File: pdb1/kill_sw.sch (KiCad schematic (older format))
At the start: 7 parts, among them P4 CONN_02X03, Q2 BUK9Y4R8-60E, U7 MIC5014, U8 NSI45020AT1G

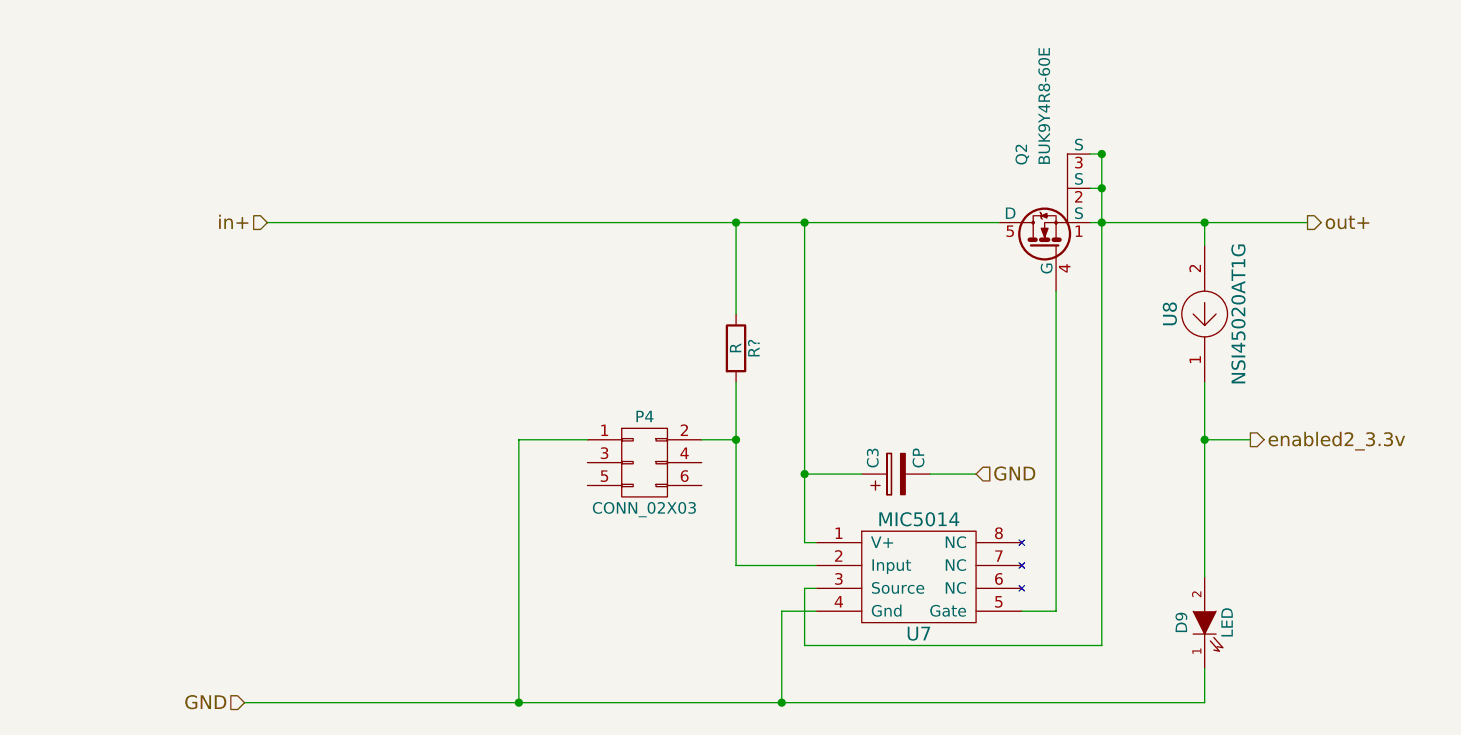
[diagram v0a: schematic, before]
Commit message: test
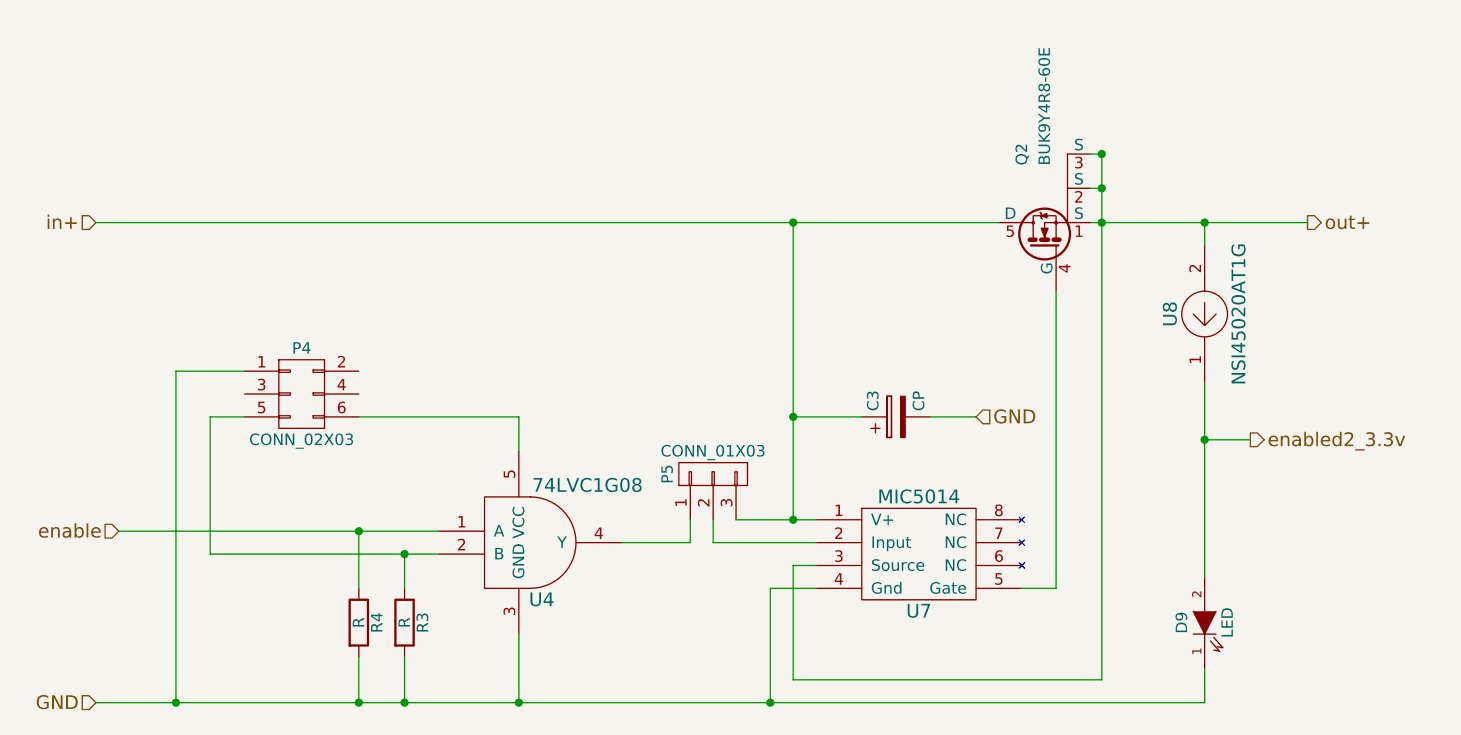
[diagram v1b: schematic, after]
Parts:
- removed R?: R, symbol R
- added P5: CONN_01X03, Pin_Headers:Pin_Header_Straight_1x03, symbol CONN_01X03
- added R3, R4: R, Resistors_SMD:R_0603, symbol R
- added U4: 74LVC1G08, TO_SOT_Packages_SMD:SOT-353, symbol 74LVC1G08
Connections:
- net GND: now also R3.2, R4.2, U4.3 (GND)
- net in+: now also P5.3 (P3)
- net at U7.2 (Input): now also P5.2 (P2); no longer P4.2 (P2)
- net at P4.5 (P5): now also R3.1, U4.2 (B)
- net at P4.6 (P6): now also U4.5 (VCC)
- new net: P5.1 (P1), U4.4 (Y)
- new net enable: R4.1, U4.1 (A)
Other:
- moved on the sheet: C3, P4, U7
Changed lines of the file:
@@
 L MIC5014 U?
 U 1 1 581F4598
-P 5250 4200
+P 5250 4100
 AR Path="/581F28FF/581F4598" Ref="U?"  Part="1"
 AR Path="/581FE101/581FE98D/581F4598" Ref="U7"  Part="1"
-F 0 "U7" H 5250 3950 60  0000 C CNN
-F 1 "MIC5014" H 5250 4450 60  0000 C CNN
-F 2 "Housings_SOIC:SOIC-8_3.9x4.9mm_Pitch1.27mm" H 5250 4100 60  0001 C CNN
-F 3 "http://www.farnell.com/datasheets/29565.pdf" H 5250 3850 60  0001 C CNN
-	1    5250 4200
-	1    0    0    -1
-$EndComp
-Text HLabel 2400 2650 0    60   Input ~ 0
+F 0 "U7" H 5250 3850 60  0000 C CNN
+F 1 "MIC5014" H 5250 4350 60  0000 C CNN
+F 2 "Housings_SOIC:SOIC-8_3.9x4.9mm_Pitch1.27mm" H 5250 4000 60  0001 C CNN
+F 3 "http://www.farnell.com/datasheets/29565.pdf" H 5250 3750 60  0001 C CNN
+	1    5250 4100
+	1    0    0    -1
+$EndComp
+Text HLabel 1650 2650 0    60   Input ~ 0
 in+
-Text HLabel 2300 4750 0    60   Input ~ 0
+Text HLabel 1650 4750 0    60   Input ~ 0
 GND
 Text HLabel 6950 2650 2    60   Output ~ 0
@@
 	0    -1   -1   0
 $EndComp
-Wire Wire Line
-	4750 4050 4800 4050
-Wire Wire Line
-	4750 2650 4750 4050
-Wire Wire Line
-	2400 2650 5600 2650
-Connection ~ 4750 2650
-Wire Wire Line
-	5850 2950 5850 4350
-Wire Wire Line
-	5850 4350 5700 4350
-Wire Wire Line
-	4650 4750 4650 4350
-Wire Wire Line
-	4650 4350 4800 4350
-Connection ~ 4650 4750
-Wire Wire Line
-	6000 2650 6950 2650
-Wire Wire Line
-	4800 4250 4750 4250
-Wire Wire Line
-	4750 4250 4750 4500
-Wire Wire Line
-	4750 4500 6050 4500
-Connection ~ 6050 2650
-Connection ~ 4750 3750
-Connection ~ 3500 4750
-Wire Wire Line
-	6500 2750 6500 2650
-Connection ~ 6500 2650
-Wire Wire Line
-	6500 4750 6500 4600
-Wire Wire Line
-	6500 3350 6500 4200
-Wire Wire Line
-	4750 3750 5000 3750
-Wire Wire Line
-	5300 3750 5500 3750
 Text HLabel 6700 3600 2    60   Output ~ 0
 enabled2_3.3v
-Wire Wire Line
-	6700 3600 6500 3600
-Connection ~ 6500 3600
-Wire Wire Line
-	2300 4750 6500 4750
-Text HLabel 5500 3750 2    60   Input ~ 0
+Text HLabel 5500 3500 2    60   Input ~ 0
 GND
 $Comp
@@
 	0    -1   -1   0
 $EndComp
+$Comp
+L CP C3
+U 1 1 5825B68F
+P 5150 3500
+F 0 "C3" H 5175 3600 50  0000 L CNN
+F 1 "CP" H 5175 3400 50  0000 L CNN
+F 2 "Capacitors_ThroughHole:C_Radial_D5_L6_P2.5" H 5188 3350 50  0001 C CNN
+F 3 "" H 5150 3500 50  0000 C CNN
+	1    5150 3500
+	0    -1   -1   0
+$EndComp
+$Comp
+L CONN_02X03 P4
+U 1 1 5825EF78
+P 2550 3400
+F 0 "P4" H 2550 3600 50  0000 C CNN
+F 1 "CONN_02X03" H 2550 3200 50  0000 C CNN
+F 2 "Pin_Headers:Pin_Header_Straight_2x03" H 2550 2200 50  0001 C CNN
+F 3 "" H 2550 2200 50  0000 C CNN
+	1    2550 3400
+	1    0    0    -1
+$EndComp
+$Comp
+L R R3
+U 1 1 582707A5
+P 3000 4400
+F 0 "R3" V 3080 4400 50  0000 C CNN
+F 1 "R" V 3000 4400 50  0000 C CNN
+F 2 "Resistors_SMD:R_0603" V 2930 4400 50  0001 C CNN
+F 3 "" H 3000 4400 50  0000 C CNN
+	1    3000 4400
+	1    0    0    -1
+$EndComp
+$Comp
+L 74LVC1G08 U4
+U 1 1 582725D8
+P 3500 4050
+F 0 "U4" H 3600 3800 60  0000 C CNN
+F 1 "74LVC1G08" H 3800 4300 60  0000 C CNN
+F 2 "TO_SOT_Packages_SMD:SOT-353" H 3450 4100 60  0001 C CNN
+F 3 "http://www.nxp.com/documents/data_sheet/74LVC1G08.pdf?" H 4000 3600 60  0001 C CNN
+	1    3500 4050
+	1    0    0    -1
+$EndComp
+Wire Wire Line
+	4450 3950 4800 3950
+Wire Wire Line
+	4700 2650 4700 3950
+Wire Wire Line
+	1650 2650 5600 2650
+Connection ~ 4700 2650
+Wire Wire Line
+	5850 2950 5850 4250
+Wire Wire Line
+	5850 4250 5700 4250
+Wire Wire Line
+	4600 4750 4600 4250
+Wire Wire Line
+	4600 4250 4800 4250
+Connection ~ 4600 4750
+Wire Wire Line
+	6000 2650 6950 2650
+Wire Wire Line
+	4800 4150 4700 4150
+Wire Wire Line
+	6050 4650 4700 4650
+Connection ~ 6050 2650
+Connection ~ 4700 3500
+Wire Wire Line
+	6500 2750 6500 2650
+Connection ~ 6500 2650
+Wire Wire Line
+	6500 4750 6500 4600
+Wire Wire Line
+	6500 3350 6500 4200
+Wire Wire Line
+	4700 3500 5000 3500
+Wire Wire Line
+	5300 3500 5500 3500
+Wire Wire Line
+	6700 3600 6500 3600
+Connection ~ 6500 3600
+Wire Wire Line
+	1650 4750 6500 4750
 Wire Wire Line
 	6000 2500 6050 2500
@@
 Connection ~ 6050 2350
 Wire Wire Line
-	6050 2350 6050 4500
-$Comp
-L CP C3
-U 1 1 5825B68F
-P 5150 3750
-F 0 "C3" H 5175 3850 50  0000 L CNN
-F 1 "CP" H 5175 3650 50  0000 L CNN
-F 2 "Capacitors_ThroughHole:C_Radial_D5_L6_P2.5" H 5188 3600 50  0001 C CNN
-F 3 "" H 5150 3750 50  0000 C CNN
-	1    5150 3750
-	0    -1   -1   0
-$EndComp
-Wire Wire Line
-	3500 3600 3500 4750
-Wire Wire Line
-	4450 4150 4800 4150
-$Comp
-L CONN_02X03 P4
-U 1 1 5825EF78
-P 4050 3700
-F 0 "P4" H 4050 3900 50  0000 C CNN
-F 1 "CONN_02X03" H 4050 3500 50  0000 C CNN
-F 2 "Pin_Headers:Pin_Header_Straight_2x03" H 4050 2500 50  0001 C CNN
-F 3 "" H 4050 2500 50  0000 C CNN
-	1    4050 3700
-	1    0    0    -1
-$EndComp
-Wire Wire Line
-	3500 3600 3800 3600
-Wire Wire Line
-	4450 3350 4450 4150
-Wire Wire Line
-	4450 3600 4300 3600
-$Comp
-L R R?
-U 1 1 5825F8D9
-P 4450 3200
-F 0 "R?" V 4530 3200 50  0000 C CNN
-F 1 "R" V 4450 3200 50  0000 C CNN
-F 2 "" V 4380 3200 50  0000 C CNN
-F 3 "" H 4450 3200 50  0000 C CNN
-	1    4450 3200
-	1    0    0    -1
-$EndComp
-Connection ~ 4450 3600
-Wire Wire Line
-	4450 3050 4450 2650
-Connection ~ 4450 2650
+	6050 2350 6050 4650
+Wire Wire Line
+	3500 3500 3500 3650
+Wire Wire Line
+	3500 4450 3500 4750
+Connection ~ 3500 4750
+Wire Wire Line
+	3000 4250 3000 4100
+Wire Wire Line
+	2150 4100 3150 4100
+Wire Wire Line
+	3000 4550 3000 4750
+Connection ~ 3000 4750
+Wire Wire Line
+	2000 3300 2000 4750
+Connection ~ 2000 4750
+Wire Wire Line
+	1750 4000 3150 4000
+Wire Wire Line
+	4700 4650 4700 4150
+$Comp
+L R R4
+U 1 1 58273070
+P 2800 4400
+F 0 "R4" V 2880 4400 50  0000 C CNN
+F 1 "R" V 2800 4400 50  0000 C CNN
+F 2 "Resistors_SMD:R_0603" V 2730 4400 50  0001 C CNN
+F 3 "" H 2800 4400 50  0000 C CNN
+	1    2800 4400
+	1    0    0    -1
+$EndComp
+Wire Wire Line
+	2800 4000 2800 4250
+Connection ~ 2800 4000
+Wire Wire Line
+	2800 4550 2800 4750
+Connection ~ 2800 4750
+Text HLabel 1750 4000 0    60   Input ~ 0
+enable
+Wire Wire Line
+	2000 3300 2300 3300
+$Comp
+L CONN_01X03 P5
+U 1 1 5827405B
+P 4350 3750
+F 0 "P5" H 4350 3950 50  0000 C CNN
+F 1 "CONN_01X03" V 4450 3750 50  0000 C CNN
+F 2 "Pin_Headers:Pin_Header_Straight_1x03" H 4350 3750 50  0001 C CNN
+F 3 "" H 4350 3750 50  0000 C CNN
+	1    4350 3750
+	0    -1   -1   0
+$EndComp
+Wire Wire Line
+	4800 4050 4350 4050
+Wire Wire Line
+	4350 4050 4350 3950
+Wire Wire Line
+	3950 4050 4250 4050
+Wire Wire Line
+	4250 4050 4250 3950
+Connection ~ 4700 3950
+Wire Wire Line
+	2800 3500 3500 3500
+Connection ~ 3000 4100
+Wire Wire Line
+	2150 4100 2150 3500
+Wire Wire Line
+	2150 3500 2300 3500
 $EndSCHEMATC
